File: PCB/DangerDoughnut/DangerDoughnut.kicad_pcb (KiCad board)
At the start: 4 copper layers, 50 x 37 mm, 120 parts, among them J1 Conn_01x02_Pin, J2 Conn_01x02_Pin, J3 Conn_01x02_Pin, J4 Conn_01x04_Pin, J5 TC2030-NL, J6 USB_C_Receptacle_USB2.0_16P, SW1 SW_Push, SW2 SW_Push, U1 MMC5983MA, U10 ESP32-S3, U2 H3LIS331DLTR, U3 H3LIS331DLTR, U4 W25X20CLZP, U6 L5973D, U7 MIC5219-3.3YM5, U8 ESP8285H16, U9 SX1280IMLTRT, Y1 40MHz, Y2 52MHz, Y3 26MHz

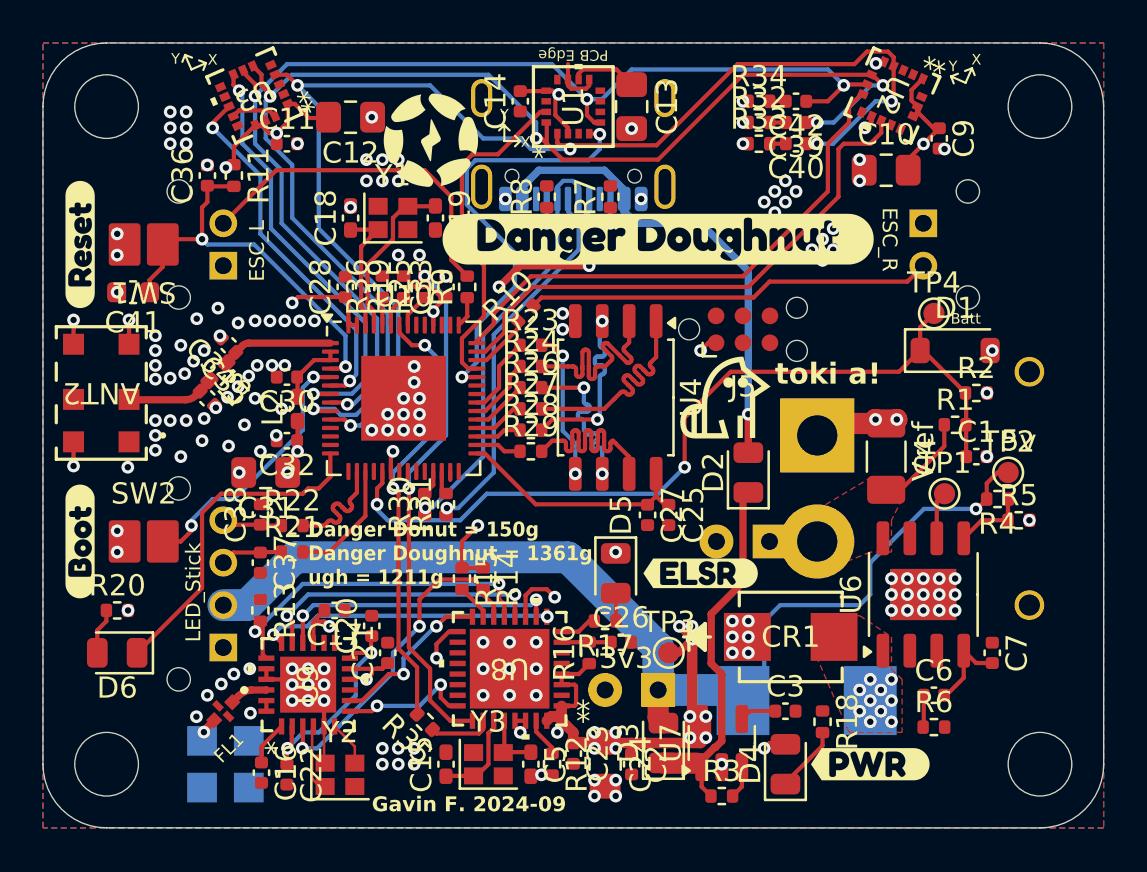
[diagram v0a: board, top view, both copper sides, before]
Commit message: test points done
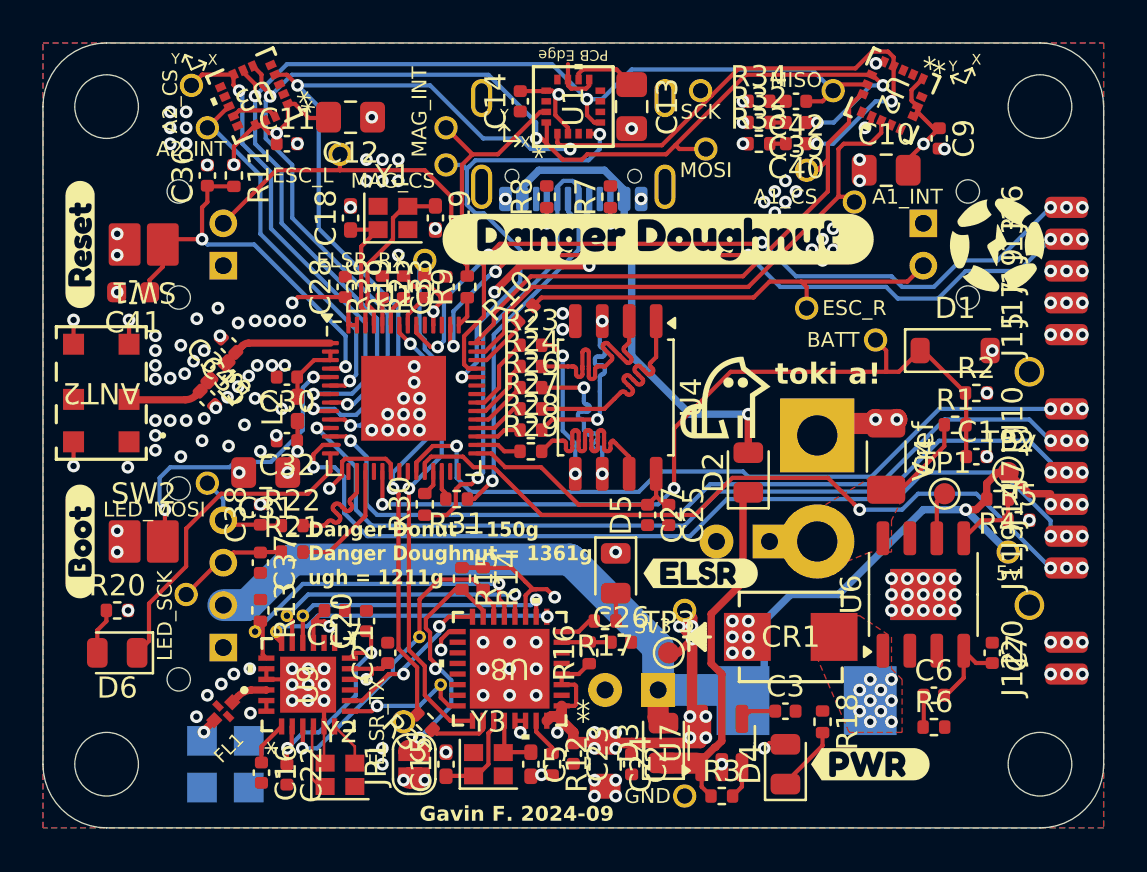
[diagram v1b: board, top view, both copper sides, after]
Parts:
- removed J5: TC2030-NL, Connector:Tag-Connect_TC2030-IDC-NL_2x03_P1.27mm_Vertical
- added J10: Conn_01x01_Pin, Connector_Wire:SolderWirePad_1x01_SMD_1x2mm, F.Cu at (123.2, 53.2)
- added J11: Conn_01x01_Pin, Connector_Wire:SolderWirePad_1x01_SMD_1x2mm, F.Cu at (123.2, 60.8)
- added J12: Conn_01x01_Pin, Connector_Wire:SolderWirePad_1x01_SMD_1x2mm, F.Cu at (123.2, 65.8)
- added J13: Conn_01x01_Pin, Connector_Wire:SolderWirePad_1x01_SMD_1x2mm, F.Cu at (123.2, 45.2)
- added J14: Conn_01x01_Pin, Connector_Wire:SolderWirePad_1x01_SMD_1x2mm, F.Cu at (123.2, 57.8)
- added J15: Conn_01x01_Pin, Connector_Wire:SolderWirePad_1x01_SMD_1x2mm, F.Cu at (123.2, 49.8)
- added J16: Conn_01x01_Pin, Connector_Wire:SolderWirePad_1x01_SMD_1x2mm, F.Cu at (123.2, 43.8)
- added J17: Conn_01x01_Pin, Connector_Wire:SolderWirePad_1x01_SMD_1x2mm, F.Cu at (123.2, 48.2)
- added J19: Conn_01x01_Pin, Connector_Wire:SolderWirePad_1x01_SMD_1x2mm, F.Cu at (123.2, 46.8)
- added J20: Conn_01x01_Pin, Connector_Wire:SolderWirePad_1x01_SMD_1x2mm, F.Cu at (123.2, 64.2)
- added J7: Conn_01x01_Pin, Connector_Wire:SolderWirePad_1x01_SMD_1x2mm, F.Cu at (123.2, 56.2)
- added J8: Conn_01x01_Pin, Connector_Wire:SolderWirePad_1x01_SMD_1x2mm, F.Cu at (123.2, 54.8)
- added J9: Conn_01x01_Pin, Connector_Wire:SolderWirePad_1x01_SMD_1x2mm, F.Cu at (123.2, 59.2)
- added JP1: SolderJumper_2_Open, Jumper:SolderJumper-2_P1.3mm_Open_RoundedPad1.0x1.5mm, F.Cu at (92.5, 70.0)
- added TP10: A1_CS, Danger_Doughnut_Lib:Test_Via, F.Cu at (111.0, 42.0)
- added TP11: A1_INT, Danger_Doughnut_Lib:Test_Via, F.Cu at (113.2, 43.5)
- added TP12: A2_CS, Danger_Doughnut_Lib:Test_Via, F.Cu at (82.0, 38.0)
- added TP13: A2_INT, Danger_Doughnut_Lib:Test_Via, F.Cu at (82.8, 40.0)
- added TP14: MAG_CS, Danger_Doughnut_Lib:Test_Via, F.Cu at (94.0, 41.8)
- added TP15: MAG_INT, Danger_Doughnut_Lib:Test_Via, F.Cu at (94.0, 40.0)
- added TP16: BATT, Danger_Doughnut_Lib:Test_Via, F.Cu at (114.2, 50.0)
- added TP17: SX_MOSI, Danger_Doughnut_Lib:Test_Via_small, F.Cu at (86.5, 63.0)
- added TP18: LED_MOSI, Danger_Doughnut_Lib:Test_Via, F.Cu at (82.8, 56.8)
- added TP19: LED_SCK, Danger_Doughnut_Lib:Test_Via, F.Cu at (81.8, 62.0)
- added TP20: ESC_L, Danger_Doughnut_Lib:Test_Via, F.Cu at (89.0, 41.2)
- added TP21: ESC_R, Danger_Doughnut_Lib:Test_Via, F.Cu at (111.0, 48.5)
- added TP22: SX_SCK, Danger_Doughnut_Lib:Test_Via_small, F.Cu at (86.0, 63.8)
- added TP23: SX_CS, Danger_Doughnut_Lib:Test_Via_small, F.Cu at (85.0, 63.8)
- added TP24: Busy, Danger_Doughnut_Lib:Test_Via_small, F.Cu at (93.8, 66.2)
- added TP25: RST, Danger_Doughnut_Lib:Test_Via_small, F.Cu at (92.8, 64.0)
- added TP26: 5v, Danger_Doughnut_Lib:Test_Via, F.Cu at (120.5, 60.0)
- added TP27: 3v3, Danger_Doughnut_Lib:Test_Via, F.Cu at (105.2, 62.8)
- added TP28: GND, Danger_Doughnut_Lib:Test_Via, F.Cu at (105.2, 71.5)
- added TP5: MISO, Danger_Doughnut_Lib:Test_Via, F.Cu at (112.2, 38.2)
- added TP6: MOSI, Danger_Doughnut_Lib:Test_Via, F.Cu at (106.2, 41.0)
- added TP7: SCK, Danger_Doughnut_Lib:Test_Via, F.Cu at (106.0, 38.2)
- added TP8: ELSR_TX, Danger_Doughnut_Lib:Test_Via, F.Cu at (92.0, 68.0)
- added TP9: ELSR_RX, Danger_Doughnut_Lib:Test_Via, F.Cu at (93.0, 46.2)
- TP4: value Batt -> SX_MISO; footprint TestPoint:TestPoint_Pad_D1.0mm -> Danger_Doughnut_Lib:Test_Via_small
- moved TP4 33.0 mm to (87.2, 63.0)
- moved R31 0.56 mm to (94.5, 57.5), turned to 180 degrees
- moved C20 0.34 mm to (90.2, 63.2)
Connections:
- TP4 pad 1: BATT -> SX_MISO
- U10 pad 11: unconnected-(U10-GPIO6-Pad11) -> Net-(J7-Pin_1)
- U10 pad 12: unconnected-(U10-GPIO7-Pad12) -> Net-(J8-Pin_1)
- U10 pad 13: unconnected-(U10-GPIO8-Pad13) -> Net-(J9-Pin_1)
- U10 pad 23: unconnected-(U10-GPIO17-Pad23) -> Net-(J10-Pin_1)
- U10 pad 24: unconnected-(U10-GPIO18-Pad24) -> Net-(J11-Pin_1)
- U10 pad 44: unconnected-(U10-MTCK-Pad44) -> Net-(J13-Pin_1)
- U10 pad 48: unconnected-(U10-MTMS-Pad48) -> Net-(J16-Pin_1)
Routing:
- net Net-(J9-Pin_1): track 0.00 -> 42.0 mm, vias 0 -> 4
- net Net-(J7-Pin_1): track 0.00 -> 40.9 mm, vias 0 -> 4
- net Net-(J8-Pin_1): track 0.00 -> 39.1 mm, vias 0 -> 4
- net Net-(J16-Pin_1): track 0.00 -> 36.2 mm, vias 0 -> 6
- net Net-(J11-Pin_1): track 0.00 -> 34.3 mm, vias 0 -> 4
- net Net-(J10-Pin_1): track 0.00 -> 34.2 mm, vias 0 -> 4
- net Net-(J13-Pin_1): track 0.00 -> 34.0 mm, vias 0 -> 6
- net GPIO0: track 1.71 -> 10.8 mm, vias 0 -> 2
- net +5V: track 50.9 -> 56.0 mm, vias 1 -> 4
- net +3.3V: track 82.3 -> 87.1 mm, vias 32 -> 36
- net Net-(J4-Pin_3): track 2.95 -> 5.32 mm
- net Accel2_CS: track 20.5 -> 22.7 mm
- net Net-(J4-Pin_4): track 2.84 -> 4.90 mm
- net Net-(U10-GPIO0): track 12.6 -> 14.3 mm
- net MAG_INT: track 16.0 -> 17.7 mm
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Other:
- board text removed: "ESC_L"
- board text removed: "ESC_R"
- board text removed: "LED_Stick"
- board text removed: "TODO: layout test points/headers"
